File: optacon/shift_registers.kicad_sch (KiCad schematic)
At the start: 3 parts, among them U1 HV528, U2 HV528

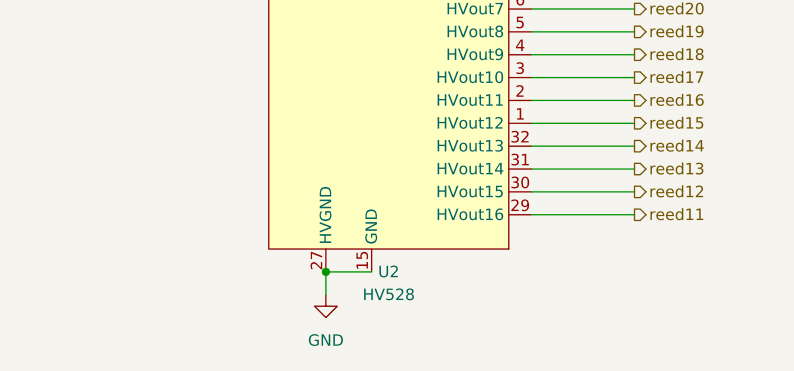
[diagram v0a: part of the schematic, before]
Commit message: test points
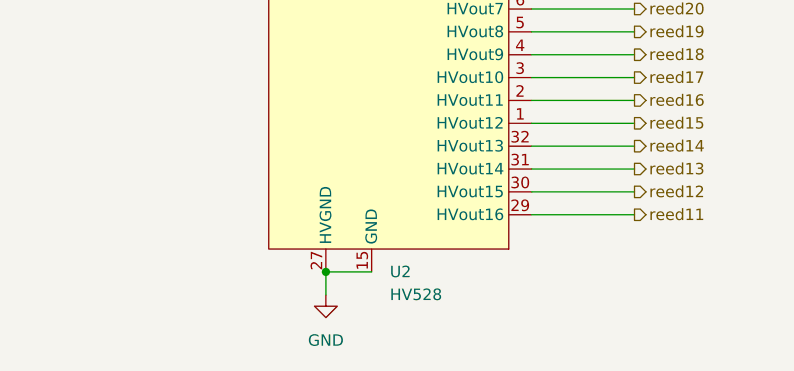
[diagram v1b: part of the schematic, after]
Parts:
- U1, U2: footprint Package_DFN_QFN:HVQFN-32-1EP_5x5mm_P0.5mm_EP3.1x3.1mm -> Package_DFN_QFN:HVQFN-32-1EP_5x5mm_P0.5mm_EP3.1x3.1mm_ThermalVias
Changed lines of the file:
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@@
       (effects (font (size 1.27 1.27)) (justify left))
     )
-    (property "Footprint" "Package_DFN_QFN:HVQFN-32-1EP_5x5mm_P0.5mm_EP3.1x3.1mm" (id 2) (at 146.05 43.18 0)
+    (property "Footprint" "Package_DFN_QFN:HVQFN-32-1EP_5x5mm_P0.5mm_EP3.1x3.1mm_ThermalVias" (id 2) (at 146.05 43.18 0)
       (effects (font (size 1.27 1.27)) hide)
     )
@@
   (symbol (lib_name "HV528_1") (lib_id "microchip_hv:HV528") (at 146.05 139.7 0) (unit 1)
     (in_bom yes) (on_board yes) (fields_autoplaced)
-    (property "Reference" "U2" (id 0) (at 145.415 168.91 0))
-    (property "Value" "HV528" (id 1) (at 145.415 171.45 0))
-    (property "Footprint" "Package_DFN_QFN:HVQFN-32-1EP_5x5mm_P0.5mm_EP3.1x3.1mm" (id 2) (at 146.05 121.92 0)
+    (property "Reference" "U2" (id 0) (at 145.5294 168.91 0)
+      (effects (font (size 1.27 1.27)) (justify left))
+    )
+    (property "Value" "HV528" (id 1) (at 145.5294 171.45 0)
+      (effects (font (size 1.27 1.27)) (justify left))
+    )
+    (property "Footprint" "Package_DFN_QFN:HVQFN-32-1EP_5x5mm_P0.5mm_EP3.1x3.1mm_ThermalVias" (id 2) (at 146.05 121.92 0)
       (effects (font (size 1.27 1.27)) hide)
     )
